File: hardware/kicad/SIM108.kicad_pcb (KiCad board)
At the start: 2 copper layers, 100 x 85 mm, 114 parts, among them J1 Screw_Terminal_01x09, J2 CAN, Q1 BC547, Q10 BC337-40, Q11 BC547, Q12 BC337-40, Q13 BC547, Q14 BC337-40, Q15 BC547, Q16 BC337-40, Q2 BC337-40, Q3 BC547, Q4 BC337-40, Q5 BC547, Q6 BC337-40, Q7 BC547, Q8 BC337-40, Q9 BC547, SW1 PRG, SW2 INSTANCE, SW3 BUS, U1 MCP2551-I-P, U10 SFH617A-1, U11 MAX6816, U12 SFH617A-1, U13 MAX6816, U14 SFH617A-1, U15 MAX6816, U16 SFH617A-1, U17 MAX6816, U18 SFH617A-1, U19 MAX6816, U2 TMR_2411, U20 SFH617A-1, U21 MAX6816, U3 MAX6816, U4 74HC595, U5 Teensy_3.2, U6 SFH617A-1, U7 MAX6816, U8 SFH617A-1, U9 MAX6816

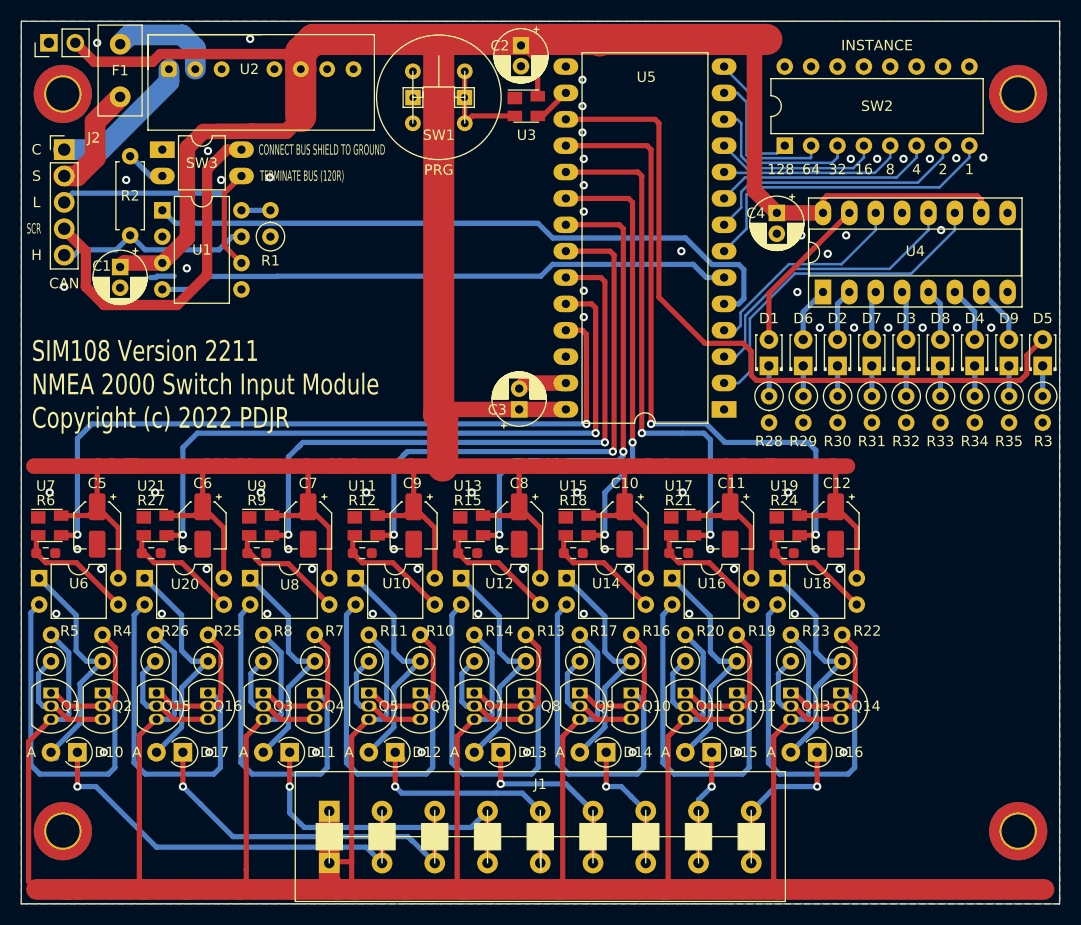
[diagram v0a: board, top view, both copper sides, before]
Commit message: PCB tweak
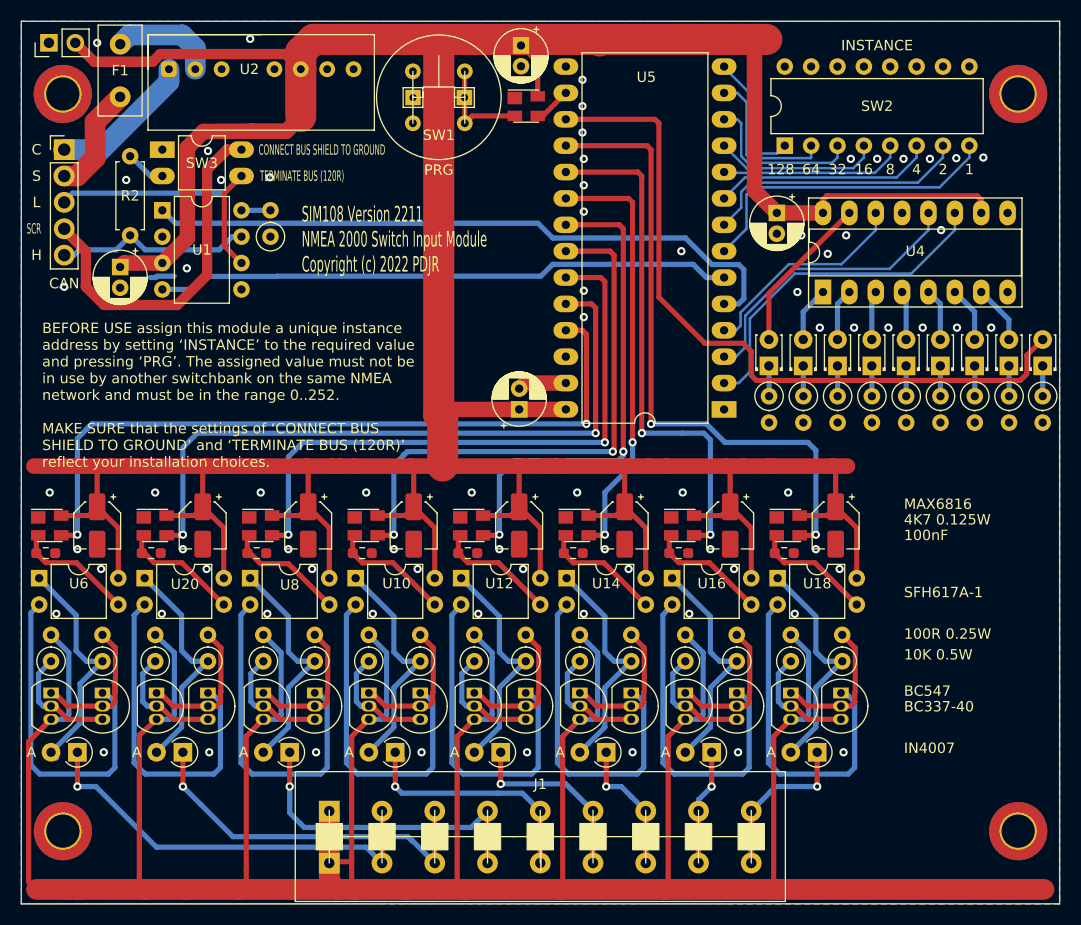
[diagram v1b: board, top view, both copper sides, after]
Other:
- board text added: "BEFORE USE assign this module a unique instance address by setting ‘INSTANCE’ to the required value and pressing ‘PRG’. The assigned value must not be in use by another switchbank on the same NMEA network and must be in the range 0..252. MAKE SURE that the settings of ‘CONNECT BUS SHIELD TO GROUND’ and ‘TERMINATE BUS (120R)’ reflect your installation choices."
